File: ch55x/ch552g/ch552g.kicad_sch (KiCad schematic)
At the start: 6 parts

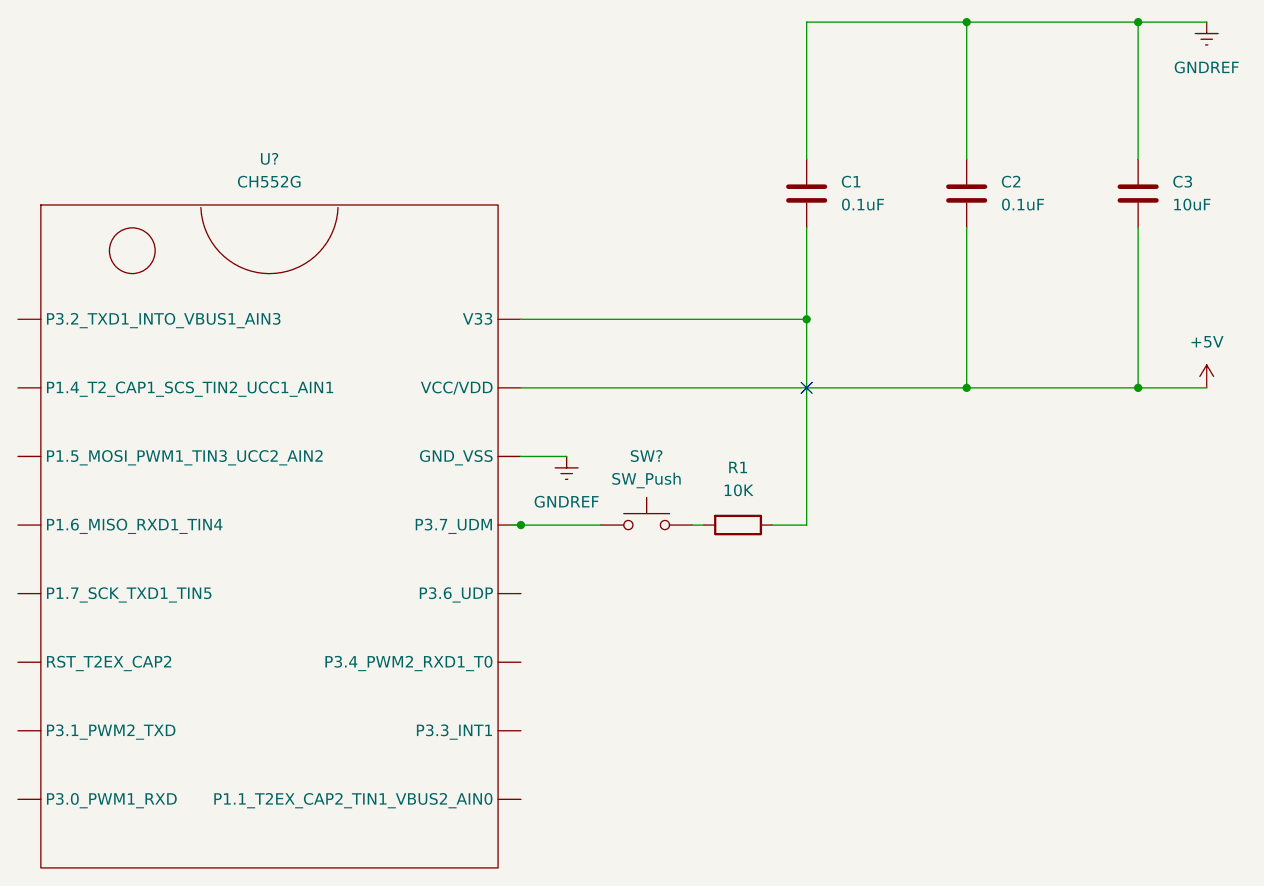
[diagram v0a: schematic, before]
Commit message: SAVE
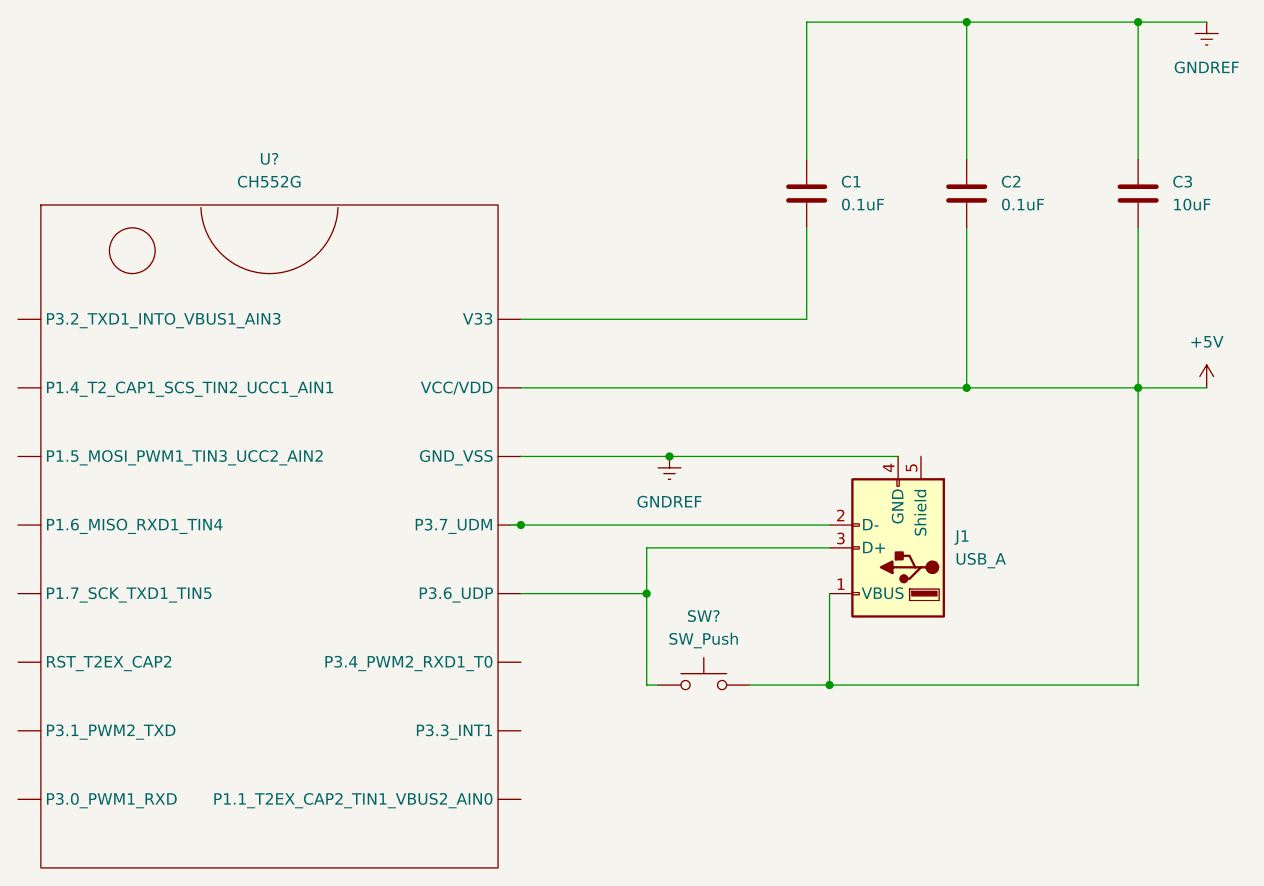
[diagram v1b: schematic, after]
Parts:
- removed R1: 10K, symbol Device:R
- added J1: USB_A, symbol Connector:USB_A
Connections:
- net +5V: now also SW?.2, J1.1 (VBUS)
- net GNDREF: now also J1.4 (GND)
- net at SW?.1, U?. (VCC/VDD): now also J1.3 (D+)
- new net: J1.2 (D-), U?. (VCC/VDD)
- no-connect marks 1 -> 0
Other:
- moved on the sheet: SW?
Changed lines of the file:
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@@
 (kicad_sch (version 20211123) (generator eeschema)
   (paper "A4")
-  (junction (at 219.71 58.42) (diameter 0) (color 0 0 0 0)
+  (junction (at 222.25 99.06) (diameter 0) (color 0 0 0 0)
   )
   (junction (at 237.49 66.04) (diameter 0) (color 0 0 0 0)
   )
+  (junction (at 204.47 73.66) (diameter 0) (color 0 0 0 0)
+  )
+  (junction (at 201.93 88.9) (diameter 0) (color 0 0 0 0)
+  )
   (junction (at 256.54 25.4) (diameter 0) (color 0 0 0 0)
   )
@@
   (junction (at 237.49 25.4) (diameter 0) (color 0 0 0 0)
   )
-  (no_connect (at 219.71 66.04))
-  (wire (pts (xy 187.96 73.66) (xy 193.04 73.66))
-    (stroke (width 0) (type default) (color 0 0 0 0))
-  )
-  (wire (pts (xy 219.71 58.42) (xy 219.71 81.28))
+  (wire (pts (xy 222.25 99.06) (xy 222.25 88.9))
+    (stroke (width 0) (type default) (color 0 0 0 0))
+  )
+  (wire (pts (xy 204.47 73.66) (xy 229.87 73.66))
+    (stroke (width 0) (type default) (color 0 0 0 0))
+  )
+  (wire (pts (xy 222.25 99.06) (xy 256.54 99.06))
+    (stroke (width 0) (type default) (color 0 0 0 0))
+  )
+  (wire (pts (xy 222.25 83.82) (xy 201.93 83.82))
+    (stroke (width 0) (type default) (color 0 0 0 0))
+  )
+  (wire (pts (xy 187.96 81.28) (xy 222.25 81.28))
     (stroke (width 0) (type default) (color 0 0 0 0))
   )
@@
     (stroke (width 0) (type default) (color 0 0 0 0))
   )
+  (wire (pts (xy 213.36 99.06) (xy 222.25 99.06))
+    (stroke (width 0) (type default) (color 0 0 0 0))
+  )
   (wire (pts (xy 256.54 25.4) (xy 237.49 25.4))
     (stroke (width 0) (type default) (color 0 0 0 0))
   )
-  (wire (pts (xy 207.01 81.28) (xy 208.28 81.28))
+  (wire (pts (xy 201.93 88.9) (xy 187.96 88.9))
     (stroke (width 0) (type default) (color 0 0 0 0))
   )
@@
     (stroke (width 0) (type default) (color 0 0 0 0))
   )
+  (wire (pts (xy 201.93 99.06) (xy 203.2 99.06))
+    (stroke (width 0) (type default) (color 0 0 0 0))
+  )
   (wire (pts (xy 256.54 66.04) (xy 264.16 66.04))
     (stroke (width 0) (type default) (color 0 0 0 0))
@@
     (stroke (width 0) (type default) (color 0 0 0 0))
   )
-  (wire (pts (xy 219.71 81.28) (xy 215.9 81.28))
+  (wire (pts (xy 201.93 88.9) (xy 201.93 99.06))
     (stroke (width 0) (type default) (color 0 0 0 0))
   )
@@
     (stroke (width 0) (type default) (color 0 0 0 0))
   )
+  (wire (pts (xy 256.54 48.26) (xy 256.54 66.04))
+    (stroke (width 0) (type default) (color 0 0 0 0))
+  )
+  (wire (pts (xy 219.71 48.26) (xy 219.71 58.42))
+    (stroke (width 0) (type default) (color 0 0 0 0))
+  )
+  (wire (pts (xy 256.54 99.06) (xy 256.54 66.04))
+    (stroke (width 0) (type default) (color 0 0 0 0))
+  )
+  (wire (pts (xy 219.71 25.4) (xy 219.71 40.64))
+    (stroke (width 0) (type default) (color 0 0 0 0))
+  )
+  (wire (pts (xy 201.93 83.82) (xy 201.93 88.9))
+    (stroke (width 0) (type default) (color 0 0 0 0))
+  )
   (wire (pts (xy 186.69 81.28) (xy 187.96 81.28))
     (stroke (width 0) (type default) (color 0 0 0 0))
   )
-  (wire (pts (xy 256.54 48.26) (xy 256.54 66.04))
-    (stroke (width 0) (type default) (color 0 0 0 0))
-  )
-  (wire (pts (xy 219.71 48.26) (xy 219.71 58.42))
-    (stroke (width 0) (type default) (color 0 0 0 0))
-  )
-  (wire (pts (xy 219.71 25.4) (xy 219.71 40.64))
-    (stroke (width 0) (type default) (color 0 0 0 0))
-  )
   (wire (pts (xy 256.54 40.64) (xy 256.54 25.4))
     (stroke (width 0) (type default) (color 0 0 0 0))
@@
     (stroke (width 0) (type default) (color 0 0 0 0))
   )
-  (wire (pts (xy 187.96 81.28) (xy 196.85 81.28))
+  (wire (pts (xy 187.96 73.66) (xy 204.47 73.66))
     (stroke (width 0) (type default) (color 0 0 0 0))
   )
@@
     (pin "2")
   )
-  (symbol (lib_id "Device:R") (at 212.09 81.28 270) (unit 1)
-    (in_bom yes) (on_board yes) (fields_autoplaced)
-    (property "Reference" "R1" (id 0) (at 212.09 74.93 90))
-    (property "Value" "10K" (id 1) (at 212.09 77.47 90))
-    (property "Footprint" "" (id 2) (at 212.09 79.502 90)
-      (effects (font (size 1.27 1.27)) hide)
-    )
-    (property "Datasheet" "~" (id 3) (at 212.09 81.28 0)
-      (effects (font (size 1.27 1.27)) hide)
-    )
-    (pin "1")
-    (pin "2")
-  )
-  (symbol (lib_id "Switch:SW_Push") (at 201.93 81.28 0) (unit 1)
-    (in_bom yes) (on_board yes) (fields_autoplaced)
-    (property "Reference" "SW?" (id 0) (at 201.93 73.66 0))
-    (property "Value" "SW_Push" (id 1) (at 201.93 76.2 0))
-    (property "Footprint" "" (id 2) (at 201.93 76.2 0)
-      (effects (font (size 1.27 1.27)) hide)
-    )
-    (property "Datasheet" "~" (id 3) (at 201.93 76.2 0)
-      (effects (font (size 1.27 1.27)) hide)
-    )
-    (pin "1")
-    (pin "2")
-  )
-  (symbol (lib_id "power:GNDREF") (at 193.04 73.66 0) (unit 1)
-    (in_bom yes) (on_board yes) (fields_autoplaced)
-    (property "Reference" "#PWR?" (id 0) (at 193.04 80.01 0)
-      (effects (font (size 1.27 1.27)) hide)
-    )
-    (property "Value" "GNDREF" (id 1) (at 193.04 78.74 0))
-    (property "Footprint" "" (id 2) (at 193.04 73.66 0)
-      (effects (font (size 1.27 1.27)) hide)
-    )
-    (property "Datasheet" "" (id 3) (at 193.04 73.66 0)
+  (symbol (lib_id "Switch:SW_Push") (at 208.28 99.06 0) (unit 1)
+    (in_bom yes) (on_board yes) (fields_autoplaced)
+    (property "Reference" "SW?" (id 0) (at 208.28 91.44 0))
+    (property "Value" "SW_Push" (id 1) (at 208.28 93.98 0))
+    (property "Footprint" "" (id 2) (at 208.28 93.98 0)
+      (effects (font (size 1.27 1.27)) hide)
+    )
+    (property "Datasheet" "~" (id 3) (at 208.28 93.98 0)
+      (effects (font (size 1.27 1.27)) hide)
+    )
+    (pin "1")
+    (pin "2")
+  )
+  (symbol (lib_id "power:GNDREF") (at 204.47 73.66 0) (unit 1)
+    (in_bom yes) (on_board yes) (fields_autoplaced)
+    (property "Reference" "#PWR?" (id 0) (at 204.47 80.01 0)
+      (effects (font (size 1.27 1.27)) hide)
+    )
+    (property "Value" "GNDREF" (id 1) (at 204.47 78.74 0))
+    (property "Footprint" "" (id 2) (at 204.47 73.66 0)
+      (effects (font (size 1.27 1.27)) hide)
+    )
+    (property "Datasheet" "" (id 3) (at 204.47 73.66 0)
       (effects (font (size 1.27 1.27)) hide)
     )
@@
     (pin "2")
   )
+  (symbol (lib_id "Connector:USB_A") (at 229.87 83.82 180) (unit 1)
+    (in_bom yes) (on_board yes) (fields_autoplaced)
+    (property "Reference" "J1" (id 0) (at 236.22 82.5499 0)
+      (effects (font (size 1.27 1.27)) (justify right))
+    )
+    (property "Value" "USB_A" (id 1) (at 236.22 85.0899 0)
+      (effects (font (size 1.27 1.27)) (justify right))
+    )
+    (property "Footprint" "" (id 2) (at 226.06 82.55 0)
+      (effects (font (size 1.27 1.27)) hide)
+    )
+    (property "Datasheet" " ~" (id 3) (at 226.06 82.55 0)
+      (effects (font (size 1.27 1.27)) hide)
+    )
+    (pin "1")
+    (pin "2")
+    (pin "3")
+    (pin "4")
+    (pin "5")
+  )
   (symbol (lib_id "power:GNDREF") (at 264.16 25.4 0) (unit 1)
     (in_bom yes) (on_board yes) (fields_autoplaced)
@@
       (reference "C3") (unit 1) (value "10uF") (footprint "")
     )
-    (path "/3ed10232-247d-4ba0-9bc0-e64146b7e0c7"
-      (reference "R1") (unit 1) (value "10K") (footprint "")
+    (path "/c0b9407c-ac63-4493-81cf-6f1deb3f1461"
+      (reference "J1") (unit 1) (value "USB_A") (footprint "")
     )
     (path "/79498666-6dc6-4229-a334-8a0ea61f2f0f"
